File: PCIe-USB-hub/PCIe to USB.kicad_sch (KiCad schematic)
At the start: 31 parts

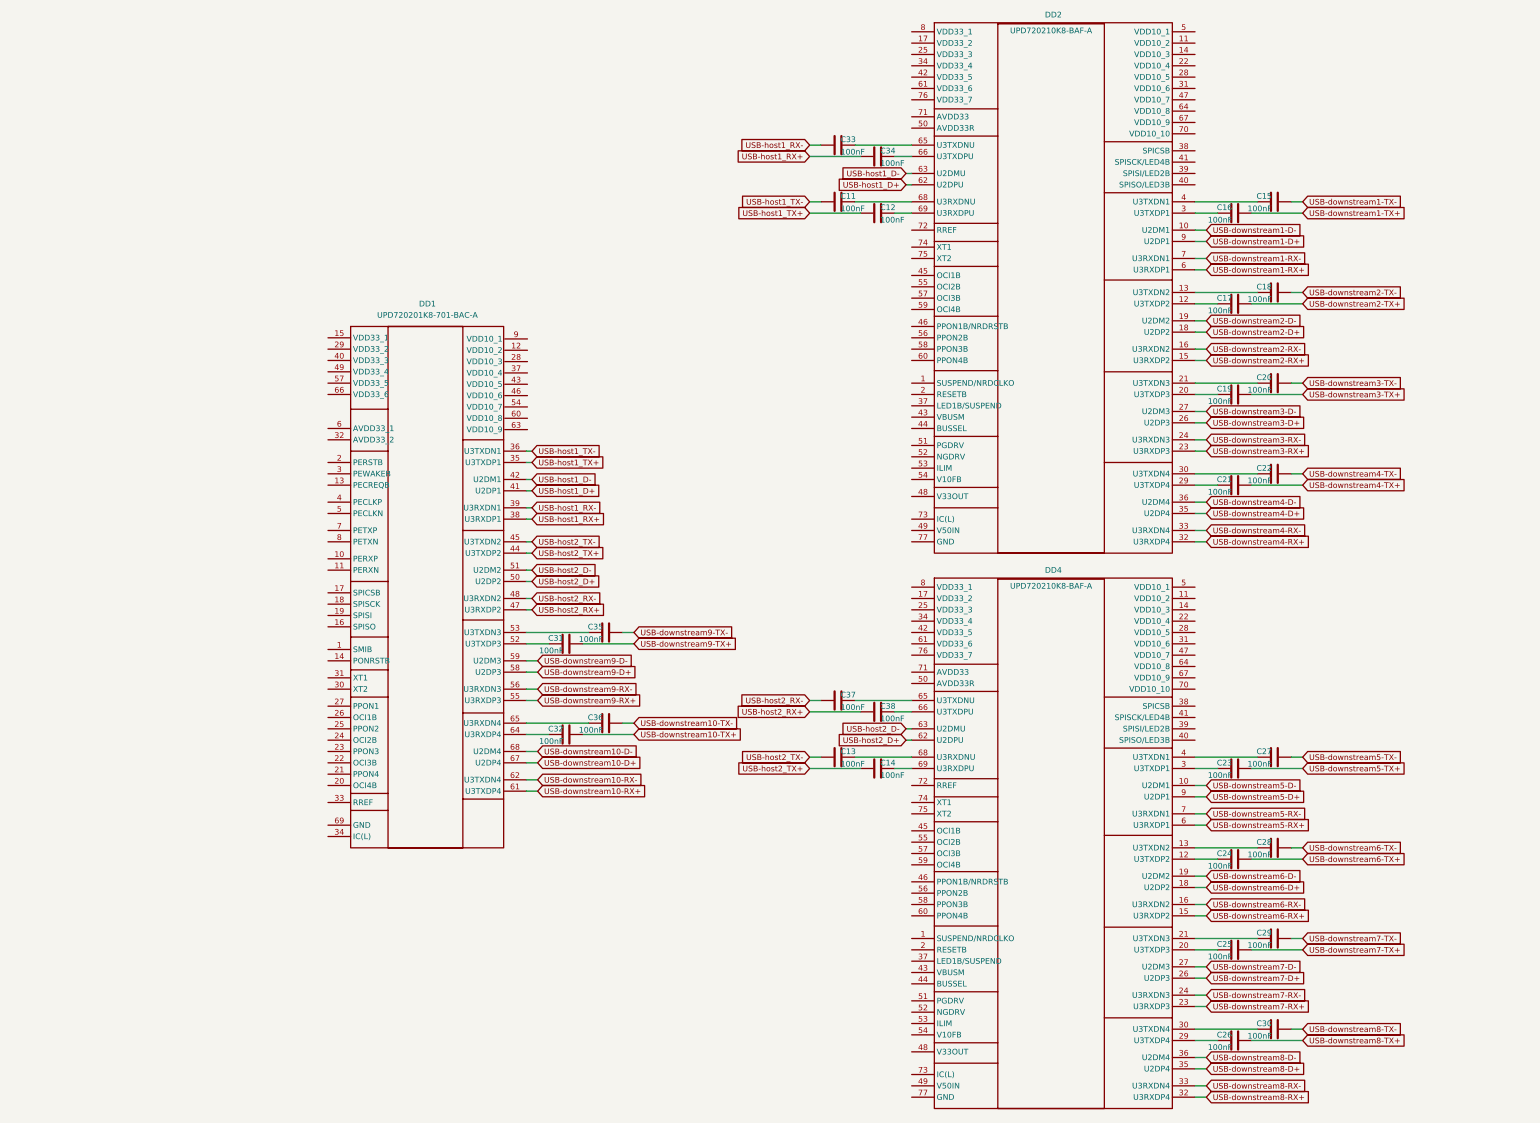
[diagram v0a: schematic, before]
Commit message: Доработка схемы, частичная конфигурация чипов
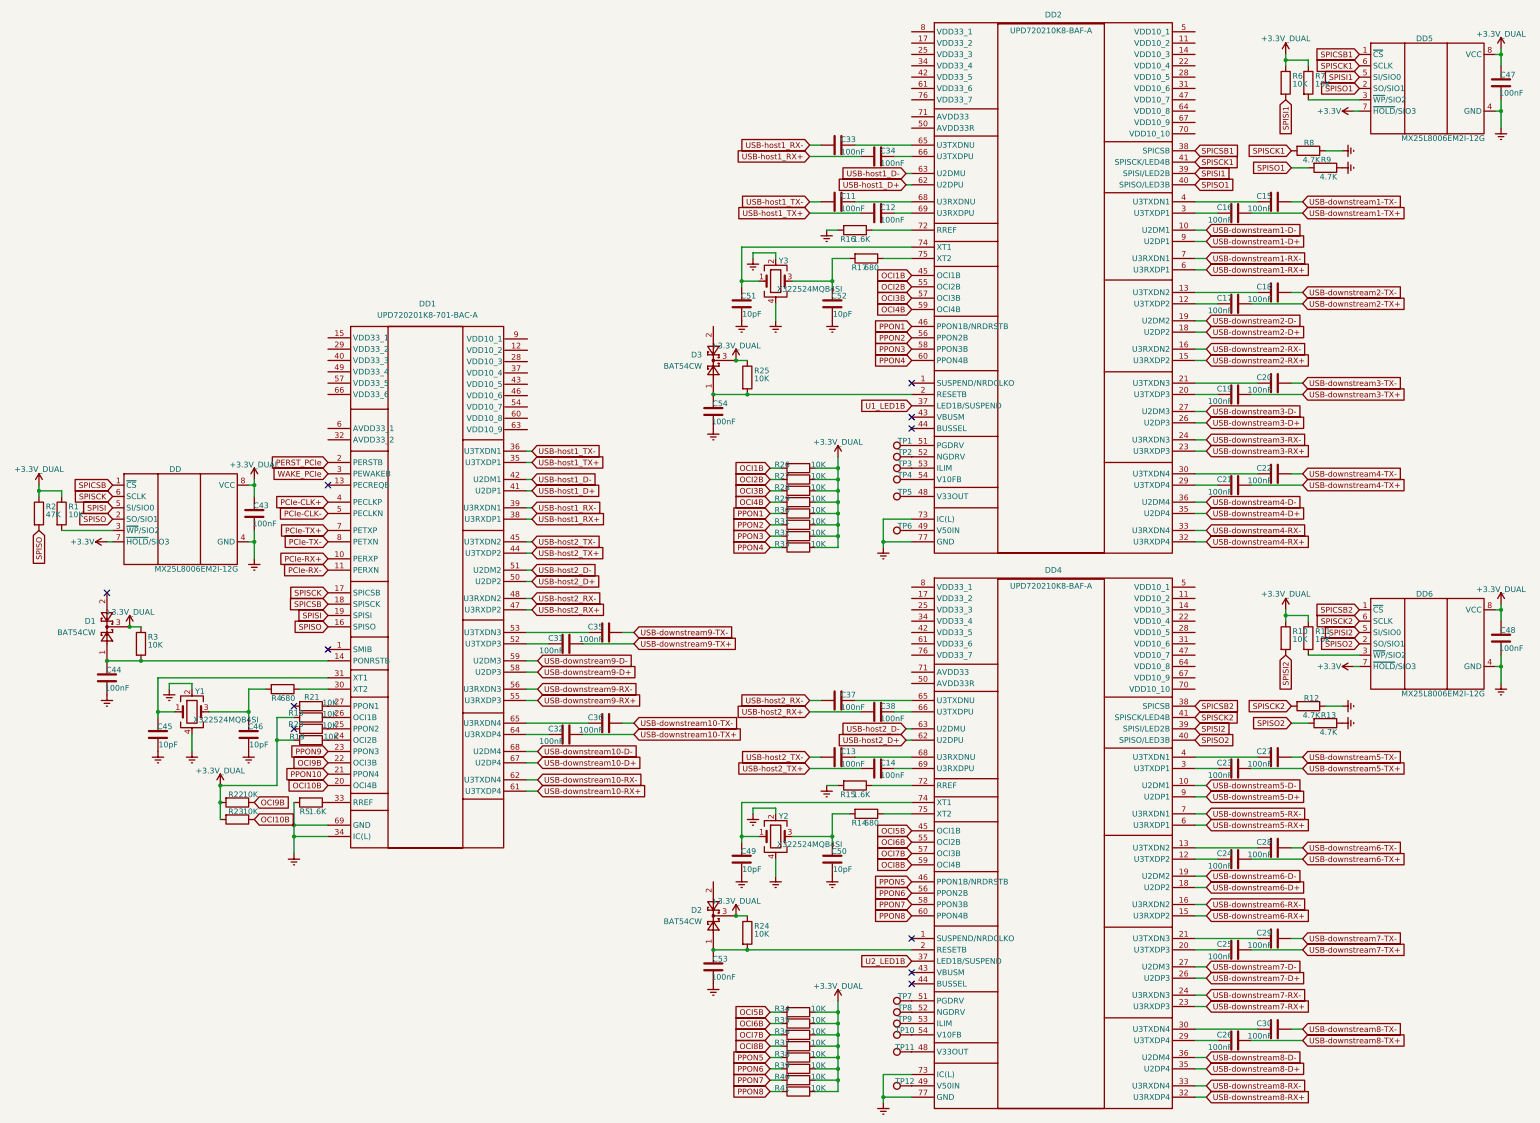
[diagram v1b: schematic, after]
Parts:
- added C43, C44, C47, C48, C53, C54: 100nF, Capacitor_SMD:C_0402_1005Metric, symbol Device:C
- added C45, C46, C49, C50, C51, C52: 10pF, Capacitor_SMD:C_0402_1005Metric, symbol Device:C
- added D1, D2, D3: BAT54CW, Package_TO_SOT_SMD:SOT-323_SC-70, symbol Diode:BAT54CW
- added DD, DD5, DD6: MX25L8006EM2I-12G, Package_SO:SOP-8_3.9x4.9mm_P1.27mm, symbol Memory_Flash:MX25L3233FM1
- added R1, R10, R11, R18, R19, R20, R21, R22, R23, R24, R25, R26, R27, R28, R29, R3, R30, R31, R32, R33, R34, R35, R36, R37, R38, R39, R40, R41, R6, R7: 10K, PCM_Resistor_SMD_AKL:R_0603_1608Metric, symbol Device:R
- added R12, R13, R8, R9: 4.7K, PCM_Resistor_SMD_AKL:R_0603_1608Metric, symbol Device:R
- added R14, R17, R4: 680, PCM_Resistor_SMD_AKL:R_0603_1608Metric, symbol Device:R
- added R15, R16, R5: 1.6K, PCM_Resistor_SMD_AKL:R_0603_1608Metric, symbol Device:R
- added R2: 47K, PCM_Resistor_SMD_AKL:R_0603_1608Metric, symbol Device:R
- added TP1, TP10, TP11, TP12, TP2, TP3, TP4, TP5, TP6, TP7, TP8, TP9: TestPoint, TestPoint:TestPoint_Pad_D1.0mm, symbol Connector:TestPoint
- added Y1, Y2, Y3: X322524MQB4SI, Crystal:Crystal_SMD_Abracon_ABM8AIG-4Pin_3.2x2.5mm, symbol Device:Crystal_GND24
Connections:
- net PCIe-RX+: now reaches DD1.10 (PERXP)
- net PCIe-RX-: now reaches DD1.11 (PERXN)
- net at DD1.14 (PONRSTB): now also C44.1, D1.1, R3.2
- net SPISO: now reaches DD1.16 (SPISO)
- net SPISO: now also DD.2 (SO/SIO1), R2.2
- net SPISCK: now reaches DD1.17 (SPICSB)
- net SPISCK: now also DD.6 (SCLK)
- net SPICSB: now reaches DD1.18 (SPISCK)
- net SPICSB: now also DD.1 (~{CS})
- net SPISI: now reaches DD1.19 (SPISI)
- net SPISI: now also DD.5 (SI/SIO0)
- net PERST_PCIe: now reaches DD1.2 (PERSTB)
- net OCI10B: now reaches DD1.20 (OCI4B)
- net OCI10B: now also R23.1
- net PPON10: now reaches DD1.21 (PPON4)
- net OCI9B: now reaches DD1.22 (OCI3B)
- net OCI9B: now also R22.1
- net PPON9: now reaches DD1.23 (PPON3)
- net at DD1.24 (OCI2B): now also R19.1
- net at DD1.25 (PPON2): now also R20.1
- net at DD1.26 (OCI1B): now also R18.1
- net at DD1.27 (PPON1): now also R21.1
- net WAKE_PCIe: now reaches DD1.3 (PEWAKEB)
- net at DD1.30 (XT2): now also R4.1
- net at DD1.31 (XT1): now also C45.1, Y1.1
- net at DD1.33 (RREF): now also R5.1
- net Earth: now reaches DD1.34 (IC(L))
- net Earth: now also DD1.69 (GND), DD2.73 (IC(L)), DD2.77 (GND), DD4.73 (IC(L)), DD4.77 (GND), C43.2, C44.2, C45.2, C46.2, C47.2, C48.2, C49.2, C50.2, C51.2, C52.2, C53.2, C54.2, DD.4 (GND), DD5.4 (GND), DD6.4 (GND), R12.1, R13.1, R15.2, R16.2, R5.2, R8.1, R9.1, Y1.2, Y1.4, Y2.2, Y2.4, Y3.2, Y3.4
- net PCIe-CLK+: now reaches DD1.4 (PECLKP)
- net PCIe-CLK-: now reaches DD1.5 (PECLKN)
- net PCIe-TX+: now reaches DD1.7 (PETXP)
- net PCIe-TX-: now reaches DD1.8 (PETXN)
- net at DD2.2 (RESETB): now also C54.1, D3.1, R25.2
- net U1_LED1B: now reaches DD2.37 (LED1B/SUSPEND)
- net SPICSB1: now reaches DD2.38 (SPICSB)
- net SPICSB1: now also DD5.1 (~{CS})
- net SPISI1: now reaches DD2.39 (SPISI/LED2B)
- net SPISI1: now also DD5.5 (SI/SIO0), R6.2
- net SPISO1: now reaches DD2.40 (SPISO/LED3B)
- net SPISO1: now also DD5.2 (SO/SIO1), R9.2
- net SPISCK1: now reaches DD2.41 (SPISCK/LED4B)
- net SPISCK1: now also DD5.6 (SCLK), R8.2
- net OCI1B: now reaches DD2.45 (OCI1B)
- net OCI1B: now also R26.2
- net PPON1: now reaches DD2.46 (PPON1B/NRDRSTB)
- net PPON1: now also R30.2
- net at DD2.48 (V33OUT): now also TP5.1
- net at DD2.49 (V50IN): now also TP6.1
- net at DD2.51 (PGDRV): now also TP1.1
- net at DD2.52 (NGDRV): now also TP2.1
- net at DD2.53 (ILIM): now also TP3.1
- net at DD2.54 (V10FB): now also TP4.1
- net OCI2B: now reaches DD2.55 (OCI2B)
- net OCI2B: now also R27.2
- net PPON2: now reaches DD2.56 (PPON2B)
- net PPON2: now also R31.2
- net OCI3B: now reaches DD2.57 (OCI3B)
- net OCI3B: now also R28.2
- net PPON3: now reaches DD2.58 (PPON3B)
- net PPON3: now also R32.2
- net OCI4B: now reaches DD2.59 (OCI4B)
- net OCI4B: now also R29.2
- net PPON4: now reaches DD2.60 (PPON4B)
- net PPON4: now also R33.2
- net at DD2.72 (RREF): now also R16.1
- net at DD2.74 (XT1): now also C51.1, Y3.1
- net at DD2.75 (XT2): now also R17.1
- net at DD4.2 (RESETB): now also C53.1, D2.1, R24.2
- net U2_LED1B: now reaches DD4.37 (LED1B/SUSPEND)
- net SPICSB2: now reaches DD4.38 (SPICSB)
- net SPICSB2: now also DD6.1 (~{CS})
- net SPISI2: now reaches DD4.39 (SPISI/LED2B)
- net SPISI2: now also DD6.5 (SI/SIO0), R10.2
- net SPISO2: now reaches DD4.40 (SPISO/LED3B)
- net SPISO2: now also DD6.2 (SO/SIO1), R13.2
- net SPISCK2: now reaches DD4.41 (SPISCK/LED4B)
- net SPISCK2: now also DD6.6 (SCLK), R12.2
- net OCI5B: now reaches DD4.45 (OCI1B)
- net OCI5B: now also R34.2
- net PPON5: now reaches DD4.46 (PPON1B/NRDRSTB)
- net PPON5: now also R38.2
- net at DD4.48 (V33OUT): now also TP11.1
- net at DD4.49 (V50IN): now also TP12.1
- net at DD4.51 (PGDRV): now also TP7.1
- net at DD4.52 (NGDRV): now also TP8.1
- net at DD4.53 (ILIM): now also TP9.1
- net at DD4.54 (V10FB): now also TP10.1
- net OCI6B: now reaches DD4.55 (OCI2B)
- net OCI6B: now also R35.2
- net PPON6: now reaches DD4.56 (PPON2B)
- net PPON6: now also R39.2
- net OCI7B: now reaches DD4.57 (OCI3B)
- net OCI7B: now also R36.2
- net PPON7: now reaches DD4.58 (PPON3B)
- net PPON7: now also R40.2
- net OCI8B: now reaches DD4.59 (OCI4B)
- net OCI8B: now also R37.2
- net PPON8: now reaches DD4.60 (PPON4B)
- net PPON8: now also R41.2
- net at DD4.72 (RREF): now also R15.1
- net at DD4.74 (XT1): now also C49.1, Y2.1
- net at DD4.75 (XT2): now also R14.1
- new net: DD5.3 (~{WP}/SIO2), R7.2
- new net: C52.1, R17.2, Y3.3
- new net: DD.3 (~{WP}/SIO2), R1.2
- new net: C46.1, R4.2, Y1.3
- new net: C50.1, R14.2, Y2.3
- new net: DD6.3 (~{WP}/SIO2), R11.2
- new net +3.3V: DD.7 (~{HOLD}/SIO3), DD5.7 (~{HOLD}/SIO3), DD6.7 (~{HOLD}/SIO3)
- new net +3.3V_DUAL: C43.1, C47.1, C48.1, D1.3, D2.3, D3.3, DD.8 (VCC), DD5.8 (VCC), DD6.8 (VCC), R1.1, R10.1, R11.1, R18.2, R19.2, R2.1, R22.2, R23.2, R24.1, R25.1, R26.1, R27.1, R28.1, R29.1, R3.1, R30.1, R31.1, R32.1, R33.1, R34.1, R35.1, R36.1, R37.1, R38.1, R39.1, R40.1, R41.1, R6.1, R7.1
- no-connect marks 0 -> 11
